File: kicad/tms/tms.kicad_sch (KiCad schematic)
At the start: 18 parts, among them J1 Conn_01x03, Q2 BT169B, SW1 SW_DIP_x01, SW2 SW_DIP_x01, SW3 SW_DIP_x01

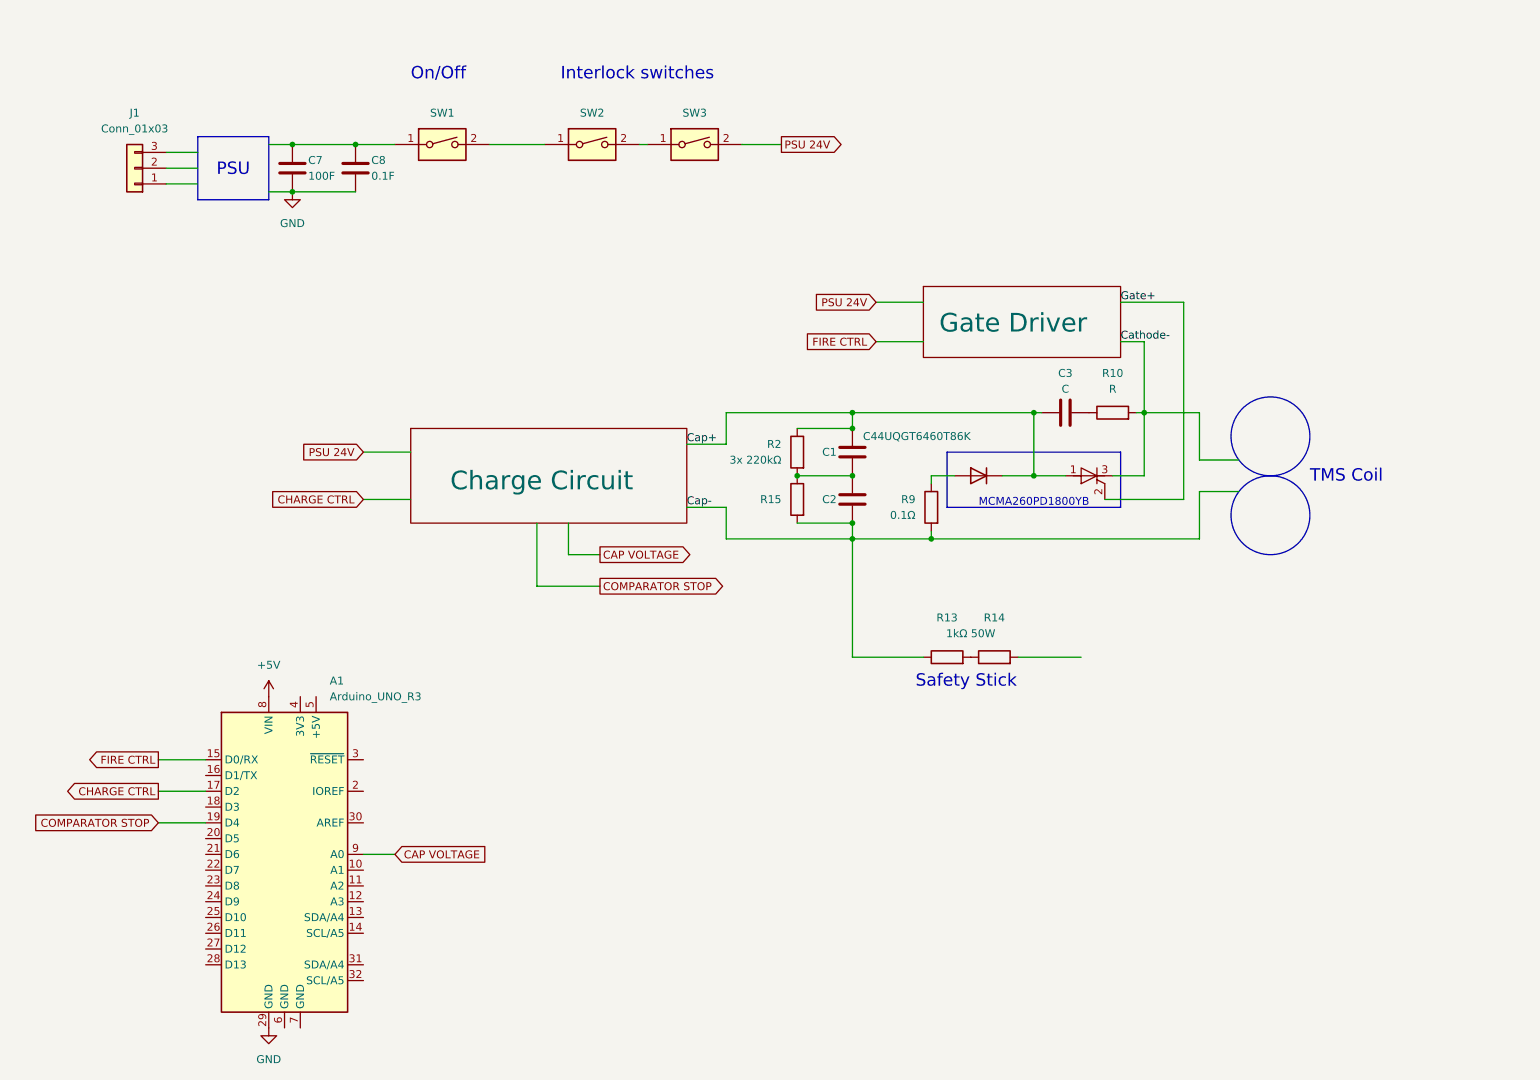
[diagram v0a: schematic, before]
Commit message: Kicad files
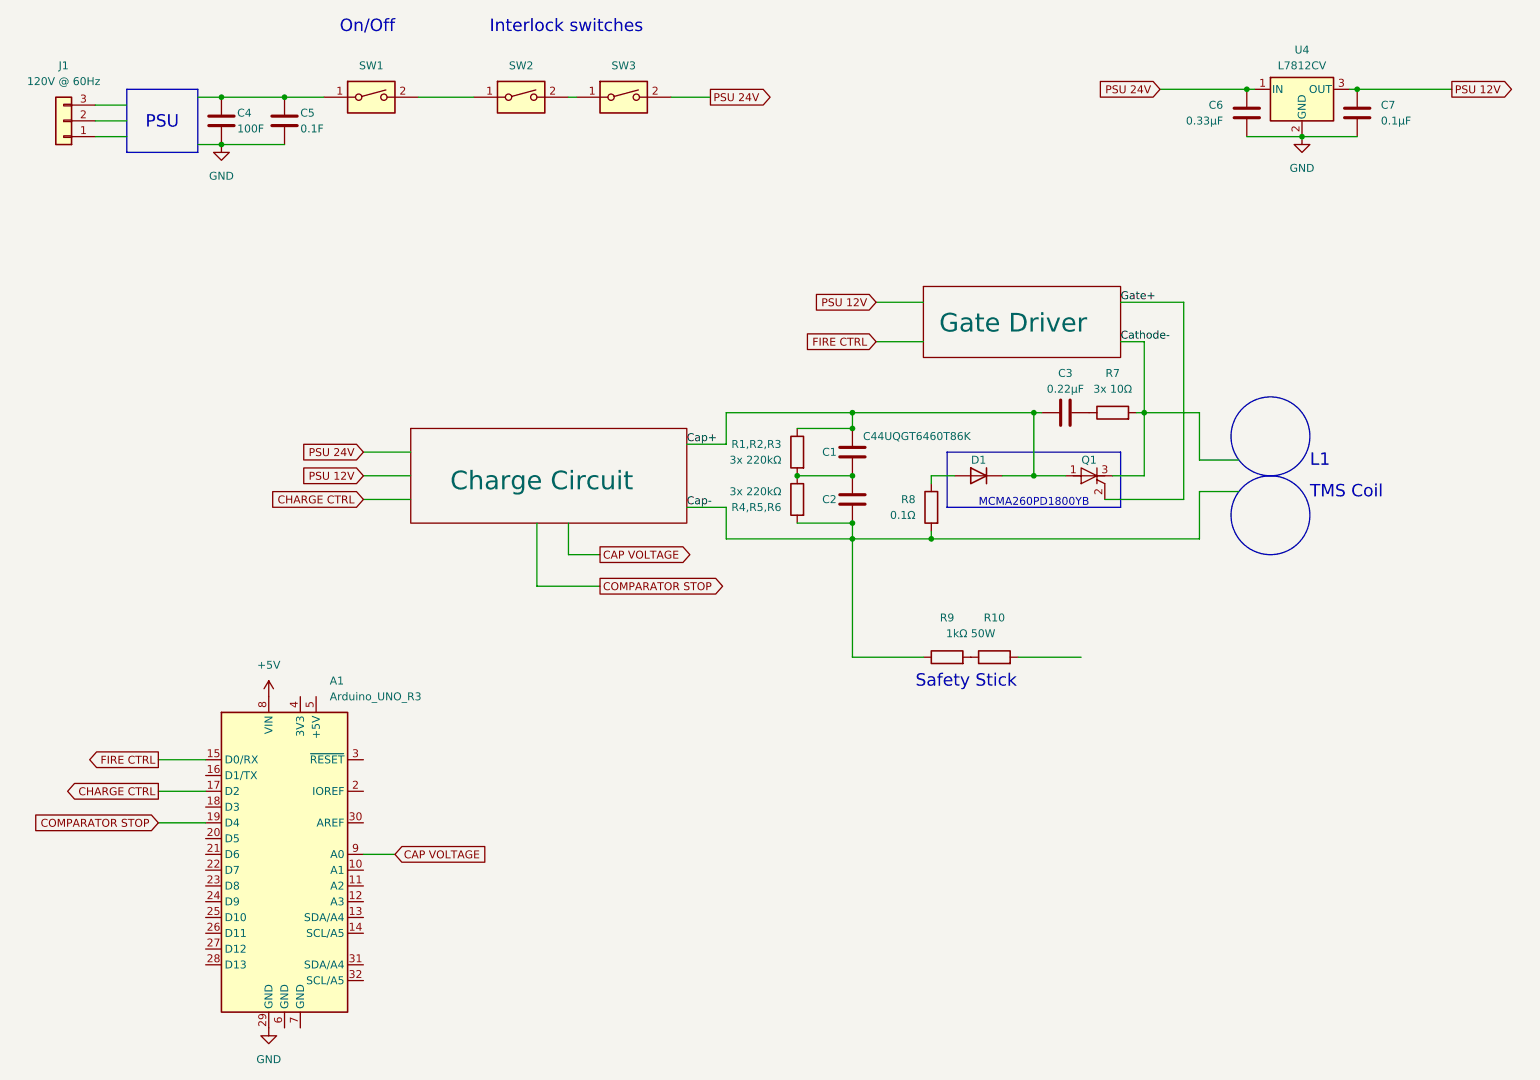
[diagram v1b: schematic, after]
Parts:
- added C6: 0.33μF, symbol Device:C
- added C7: 0.1μF, symbol Device:C
- added U4: L7812CV, symbol Regulator_Linear:L7812
- C3: value C -> 0.22μF
- J1: value Conn_01x03 -> 120V @ 60Hz
- R7: renamed from R10; value R -> 3x 10Ω
- renumbered C7 to C4, C8 to C5, D18 to D1, Q2 to Q1, R2 to R1,R2,R3, R14 to R10, R15 to R4,R5,R6, R9 to R8, R13 to R9
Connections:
- net GND: now also C6.2, C7.2, U4.2 (GND)
- net PSU 24V: now also C6.1, U4.1 (IN)
- new net PSU 12V: C7.1, U4.3 (OUT)
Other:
- note added: "L1"
- moved on the sheet: C4, C5, J1, SW1, SW2, SW3
